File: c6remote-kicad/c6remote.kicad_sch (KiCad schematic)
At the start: 24 parts, among them J1 Battery, Q1 MMBT2222A, SW1 SW_Push, SW10 SW_Push, SW11 SW_Push, SW2 SW_Push, SW3 SW_Push, SW4 SW_Push, SW5 SW_Push, SW6 SW_Push, SW7 SW_Push, SW8 SW_Push, SW9 SW_Push, U1 XIAO-ESP32-C6, U2 TSOP45xx, U3 PCF8575DBR

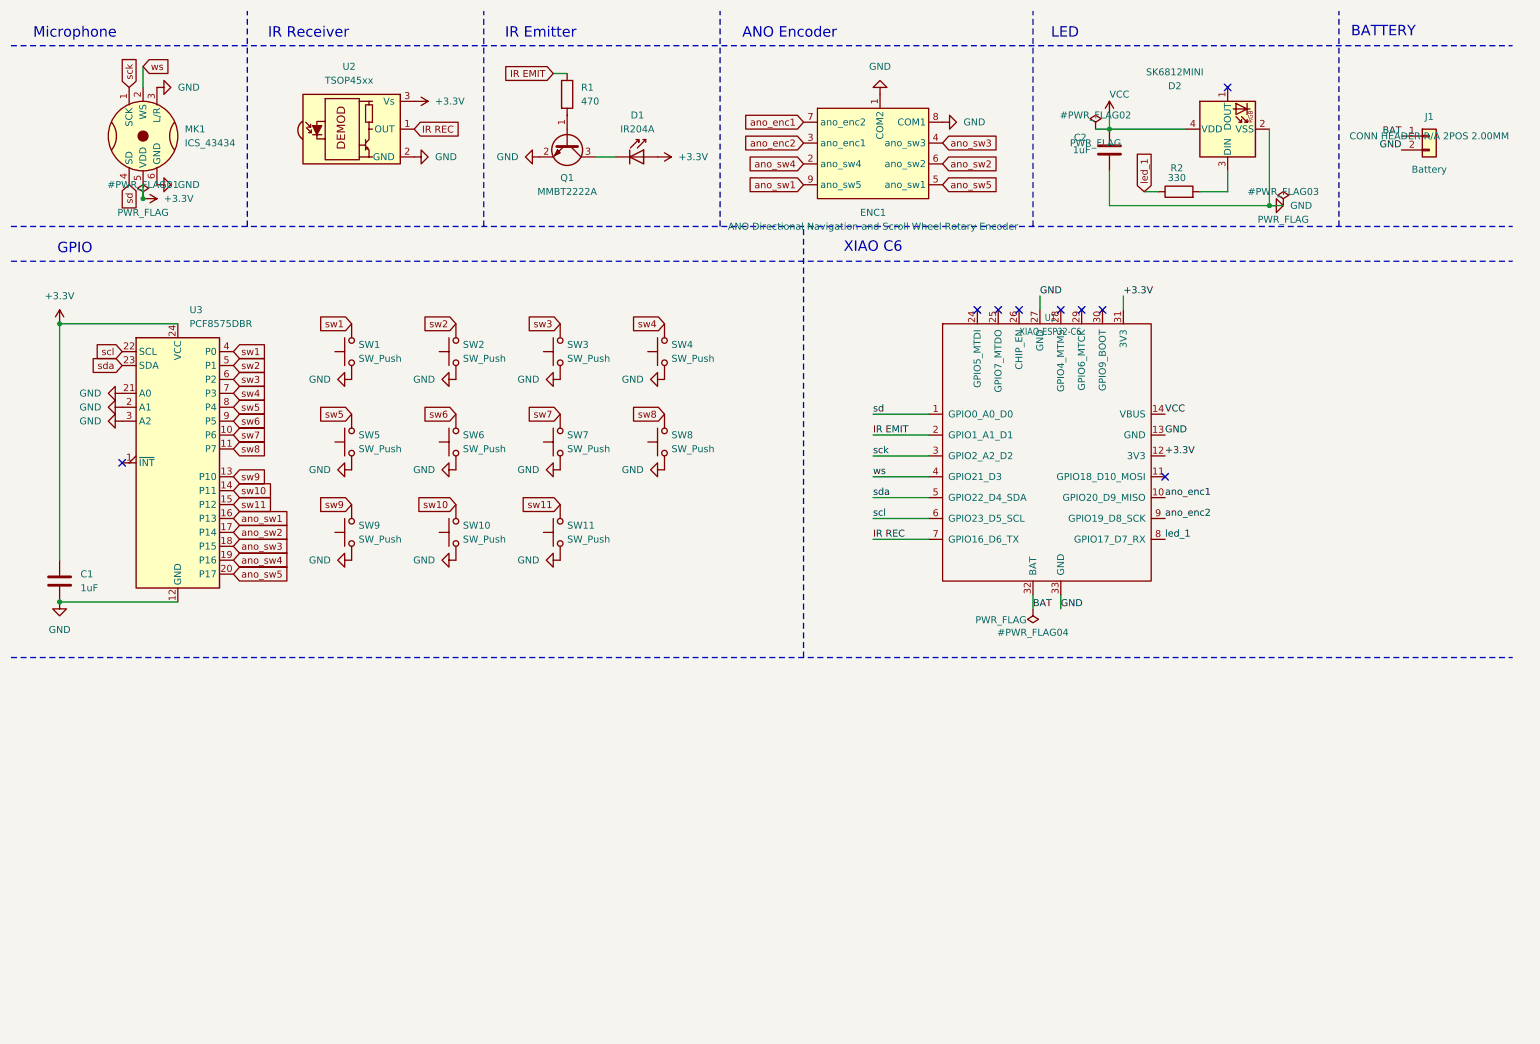
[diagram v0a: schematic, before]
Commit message: chore(assets): regenerate readme previews
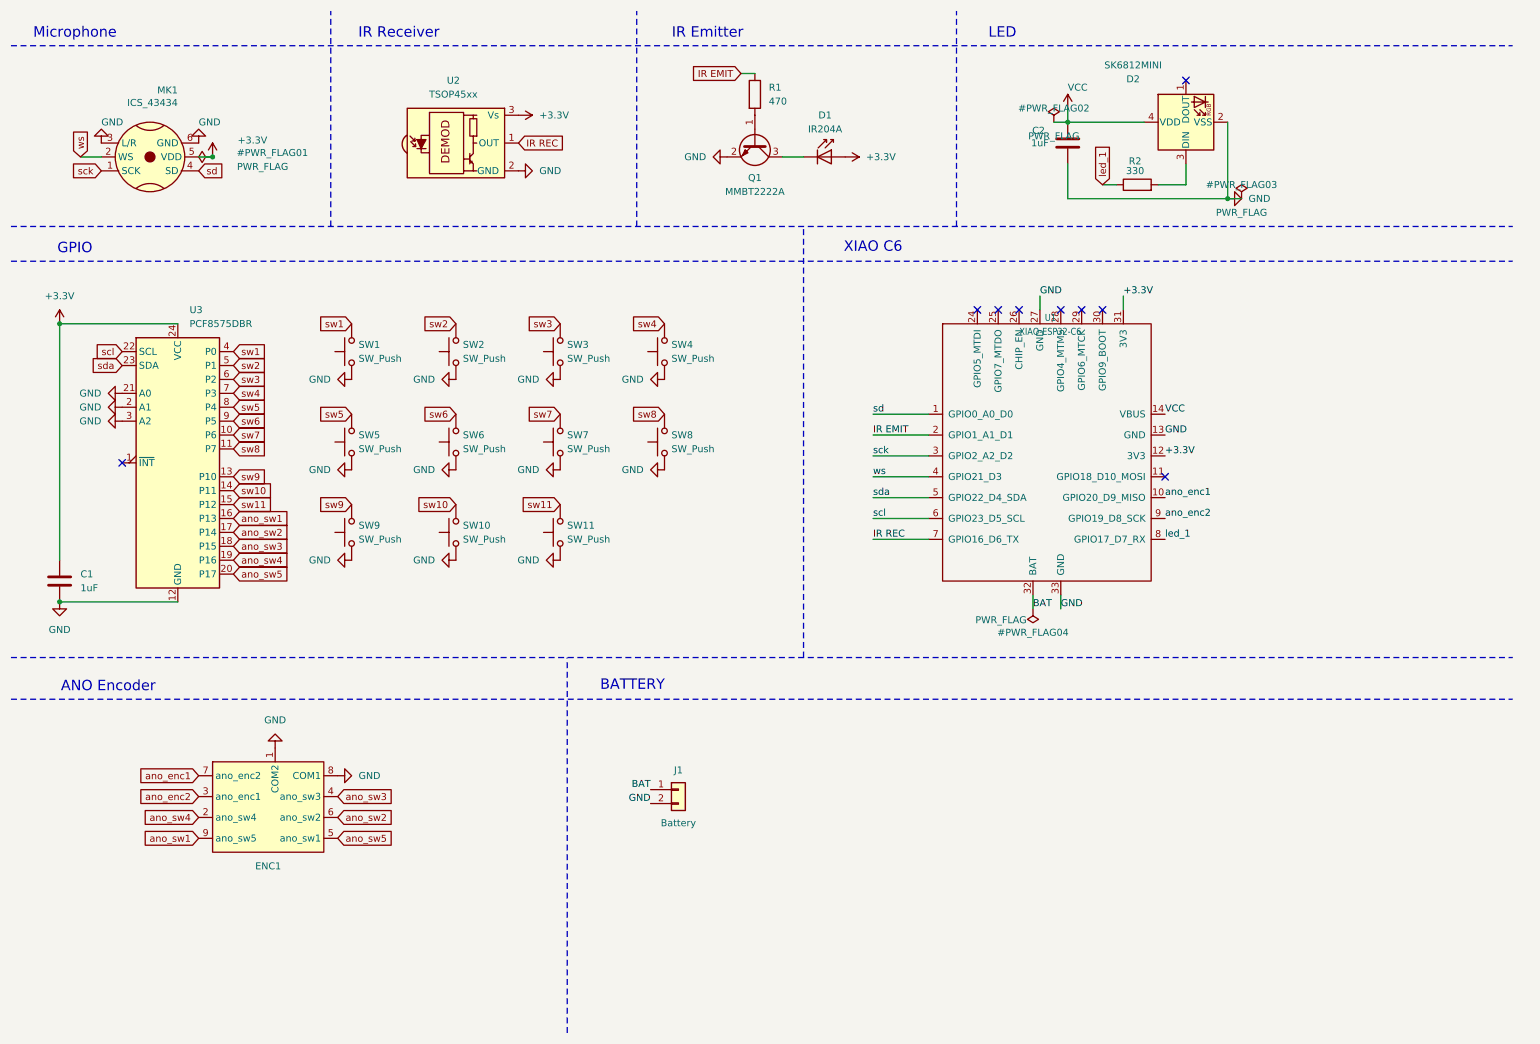
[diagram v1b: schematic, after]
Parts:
- C1, C2: MPN GRM21BR71A105MA01L -> (none); Manufacturer Murata Electronics -> (none); SKU 490-GRM21BR71A105MA01LCT-ND -> (none)
- D1: MPN IR204-A -> (none); Manufacturer Everlight Electronics Co Ltd -> (none); SKU 1080-1075-ND -> (none)
- D2: MPN 2686 -> (none); Manufacturer Adafruit Industries LLC -> (none); SKU 1528-1541-ND -> (none)
- ENC1: value ANO Directional Navigation and Scroll Wheel Rotary Encoder -> (none); MPN 5001 -> (none); Manufacturer Adafruit -> (none); SKU 5001 -> (none)
- J1: MPN S2B-PH-K-S(LF)(SN) -> (none); Manufacturer JST Sales America Inc. -> (none); SKU 455-1719-ND -> (none)
- MK1: MPN ICS-43434 -> (none); Manufacturer TDK InvenSense -> (none); SKU 1428-1066-1-ND -> (none)
- Q1: MPN MMBT2222A,215 -> (none); Manufacturer Nexperia USA Inc. -> (none); SKU 1727-4043-1-ND -> (none)
- R1: MPN RC0603FR-07470RL -> (none); Manufacturer YAGEO -> (none); SKU 311-470HRCT-ND -> (none)
- R2: MPN RC0603FR-07330RL -> (none); Manufacturer YAGEO -> (none); SKU 311-330HRCT-ND -> (none)
- SW1, SW10, SW11, SW2, SW3, SW4, SW5, SW6, SW7, SW8, SW9: MPN TL3315NF160Q -> (none); Manufacturer E-Switch -> (none); SKU EG4621CT-ND -> (none)
- U1: MPN 113991254 -> (none); Manufacturer Seeed Technology Co., Ltd -> (none); SKU 1597-113991254-ND -> XIAO-DIP
- U2: MPN TSOP4536 -> (none); Manufacturer Vishay Semiconductor Opto Division -> (none); SKU TSOP4536-ND -> (none)
- U3: MPN PCF8575DBR -> (none); Manufacturer Texas Instruments -> (none); SKU 296-17856-1-ND -> (none)
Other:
- moved on the sheet: C2, D1, D2, ENC1, J1, MK1, Q1, R1, R2, U2
